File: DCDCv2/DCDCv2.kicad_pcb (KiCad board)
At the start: 2 copper layers, 49 parts, among them M1 CSD18513Q5A, M3 CSD18533Q5A, M3_2 CSD18533Q5A, M4 CSD19534Q5A, M4_2 CSD19534Q5A, U1 LM5175PWPR

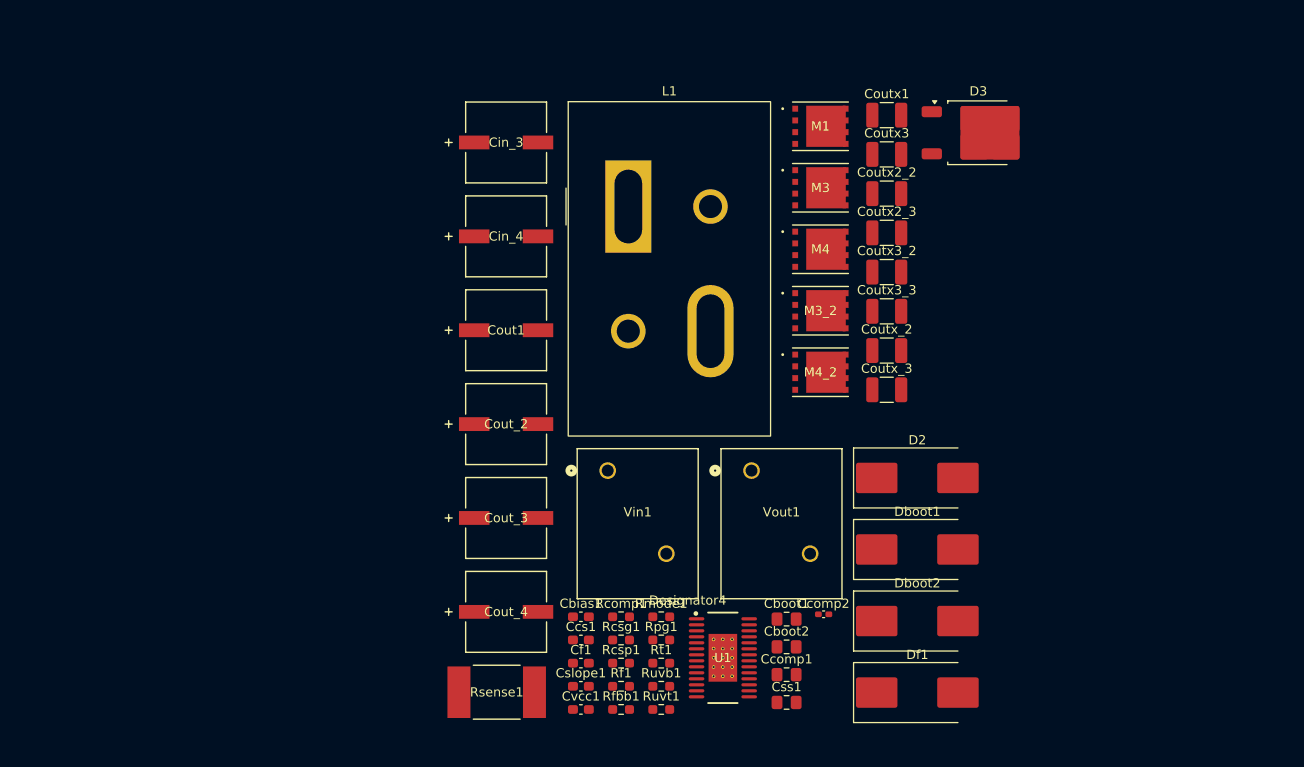
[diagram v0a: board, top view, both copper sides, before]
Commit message: preliminary pcb layout finished
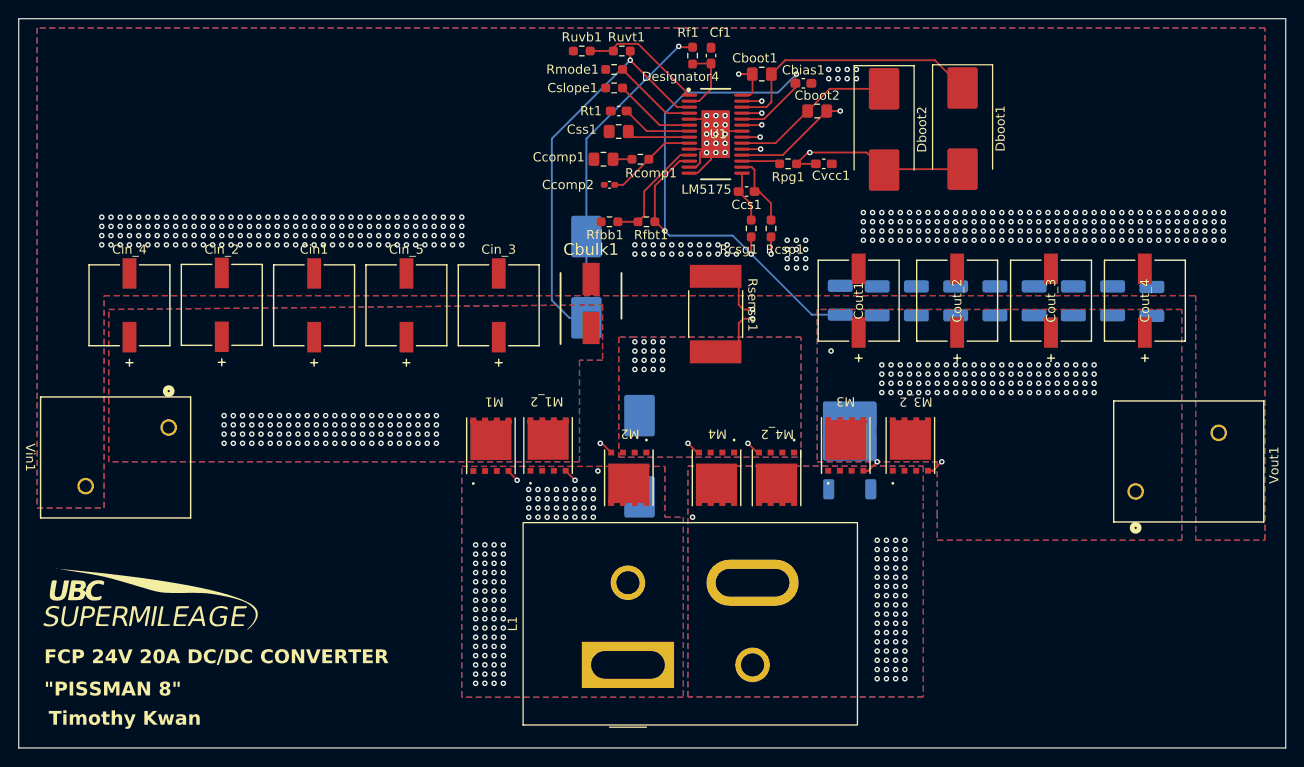
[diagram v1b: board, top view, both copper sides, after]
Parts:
- added Cbulk1: UUD1V680MCL1GS, cap footprints:CAPAE660X800N, F.Cu at (80.2, 59.9)
- added Cin1: 50SVPF39M, cap footprints:PCAP_SVP_E12_PAN, F.Cu at (50.2, 60.0)
- added Cin_2: 50SVPF39M, cap footprints:PCAP_SVP_E12_PAN, F.Cu at (40.2, 60.0)
- added Cin_5: 50SVPF39M, cap footprints:PCAP_SVP_E12_PAN, F.Cu at (60.2, 60.0)
- added Coutx2: C5750X7R2E684M, Capacitor_SMD:C_1210_3225Metric_Pad1.33x2.70mm_HandSolder, B.Cu at (107.2, 59.5)
- added G***: LOGO, logo:logo, F.Cu at (32.5, 92.0)
- added M1_2: CSD18513Q5A, CSD18531Q5A footprint:8power tdfn, F.Cu at (75.6, 75.2)
- added M2: CSD18531Q5A, CSD18531Q5A footprint:8power tdfn, F.Cu at (84.3, 78.7)
- added Rfbt1: RC0603FR-07576KL, Resistor_SMD:R_0603_1608Metric_Pad0.98x0.95mm_HandSolder, F.Cu at (86.2, 51.0)
- Cin_3, Cin_4: footprint cap footprints:35SVPF82M -> cap footprints:PCAP_SVP_E12_PAN
- Coutx1, Coutx2_2, Coutx2_3, Coutx3, Coutx3_2, Coutx3_3, Coutx_2, Coutx_3, D2, D3, Df1: moved to B.Cu
- moved Cout_4 77.0 mm to (140.2, 59.5), turned to 90 degrees
- moved Ruvt1 71.5 mm to (83.6, 32.5), turned to 180 degrees
- moved Ruvb1 69.4 mm to (79.2, 32.5), turned to 180 degrees
- moved Rf1 68.8 mm to (91.2, 33.0), turned to -90 degrees
- moved Cf1 67.3 mm to (93.2, 33.0), turned to 90 degrees
- moved Cvcc1 64.7 mm to (105.5, 44.7)
- moved Css1 64.5 mm to (83.2, 41.2), turned to 180 degrees
- moved Cout_3 63.6 mm to (130.1, 59.5), turned to 90 degrees
- moved Vin1 63.5 mm to (25.5, 79.8), turned to -90 degrees
- moved Cbias1 62.6 mm to (103.2, 36.0)
- moved Rt1 62.5 mm to (82.8, 36.5), turned to 180 degrees
- moved Cslope1 62.5 mm to (83.2, 39.0), turned to 180 degrees
- moved Rmode1 59.5 mm to (82.8, 34.5), turned to 180 degrees
- moved Ccomp1 59.3 mm to (81.6, 44.2), turned to 180 degrees
- moved Cboot1 59.1 mm to (98.8, 35.0), turned to 180 degrees
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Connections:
- Cbias1 pad 1: Net-(Cout1-+) -> Vout
- Cin_3 pad 1: Net-(Cbulk1-+) -> Vin
- Cin_4 pad 1: Net-(Cbulk1-+) -> Vin
- Cout1 pad 1: Net-(Cout1-+) -> Vout
- Cout_2 pad 1: Net-(Cout1-+) -> Vout
- Cout_3 pad 1: Net-(Cout1-+) -> Vout
- Cout_4 pad 1: Net-(Cout1-+) -> Vout
- Coutx1 pad 1: Net-(Cout1-+) -> Vout
- Coutx2_2 pad 1: Net-(Cout1-+) -> Vout
- Coutx2_3 pad 1: Net-(Cout1-+) -> Vout
- Coutx3 pad 1: Net-(Cout1-+) -> Vout
- Coutx3_2 pad 1: Net-(Cout1-+) -> Vout
- Coutx3_3 pad 1: Net-(Cout1-+) -> Vout
- Coutx_2 pad 1: Net-(Cout1-+) -> Vout
- Coutx_3 pad 1: Net-(Cout1-+) -> Vout
- D3 pad 2: Net-(Cout1-+) -> Vout
- Df1 pad 2: Net-(Cbulk1-+) -> Vin
- M1 pad 5: Net-(Cbulk1-+) -> Vin
- M3 pad 5: Net-(Cout1-+) -> Vout
- M3_2 pad 5: Net-(Cout1-+) -> Vout
- Ruvt1 pad 1: Net-(Cbulk1-+) -> Vin
- U1 pad 12: Net-(Cout1-+) -> Vout
- U1 pad 24: Net-(Cout1-+) -> Vout
- U1 pad 3: Net-(Cbulk1-+) -> Vin
- Vin1 pad 1: Net-(Cbulk1-+) -> Vin
- Vout1 pad 1: Net-(Cout1-+) -> Vout
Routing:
- net /sw2: track 0.00 -> 88.0 mm, vias 0 -> 66
- net Vout: track 0.00 -> 70.5 mm, vias 0 -> 99
- net /hdrv1: track 0.00 -> 68.8 mm, vias 0 -> 3
- net /hdrv2: track 0.00 -> 56.5 mm, vias 0 -> 3
- net /ldrv1: track 0.00 -> 55.5 mm, vias 0 -> 2
- net /sw1: track 0.00 -> 54.8 mm, vias 0 -> 98
- net /ldrv2: track 0.00 -> 54.1 mm, vias 0 -> 3
- net Vin: track 0.00 -> 44.4 mm, vias 0 -> 97
- net GND: track 0.00 -> 33.1 mm, vias 0 -> 380
- net Net-(Dboot1-A): track 0.00 -> 30.0 mm, vias 0 -> 2
- net Net-(Df1-K): track 0.00 -> 29.3 mm, vias 0 -> 1
- net Net-(Dboot1-K): track 0.00 -> 29.0 mm
- net /rcs2: track 0.00 -> 17.9 mm, vias 0 -> 18
- net Net-(Dboot2-K): track 0.00 -> 17.8 mm
- net Net-(U1-EN): track 0.00 -> 13.4 mm
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- added copper zone on B.Cu, net /rcs2
- added copper zone on F.Cu, net /rcs2
- added copper zone on B.Cu, net /sw1
- added copper zone on F.Cu, net /sw1
- added copper zone on In1.Cu, net /sw1
- added copper zone on In2.Cu, net /sw1
- added copper zone on B.Cu, net /sw2
- added copper zone on F.Cu, net /sw2
- added copper zone on In1.Cu, net /sw2
- added copper zone on In2.Cu, net /sw2
- added copper zone on B.Cu, net GND
- added copper zone on F.Cu, net GND
- added copper zone on In1.Cu, net GND
- added copper zone on In2.Cu, net GND
- added copper zone on B.Cu, net Vin
- added copper zone on F.Cu, net Vin
- added copper zone on In1.Cu, net Vin
- added copper zone on In2.Cu, net Vin
- added copper zone on B.Cu, net Vout
- added copper zone on F.Cu, net Vout
- added copper zone on In1.Cu, net Vout
- added copper zone on In2.Cu, net Vout
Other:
- board outline added: 137.2 x 79 mm
- copper layers 2 -> 4
- board text added: "FCP 24V 20A DC/DC CONVERTER"
- board text added: "Timothy Kwan"
- board text added: "{dblquote}PISSMAN 8{dblquote}"
